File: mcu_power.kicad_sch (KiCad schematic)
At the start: 36 parts, among them U1 MIMXRT1052CVJ5B, Y1 DSC1001BI5-024.0000, Y2 830107834801

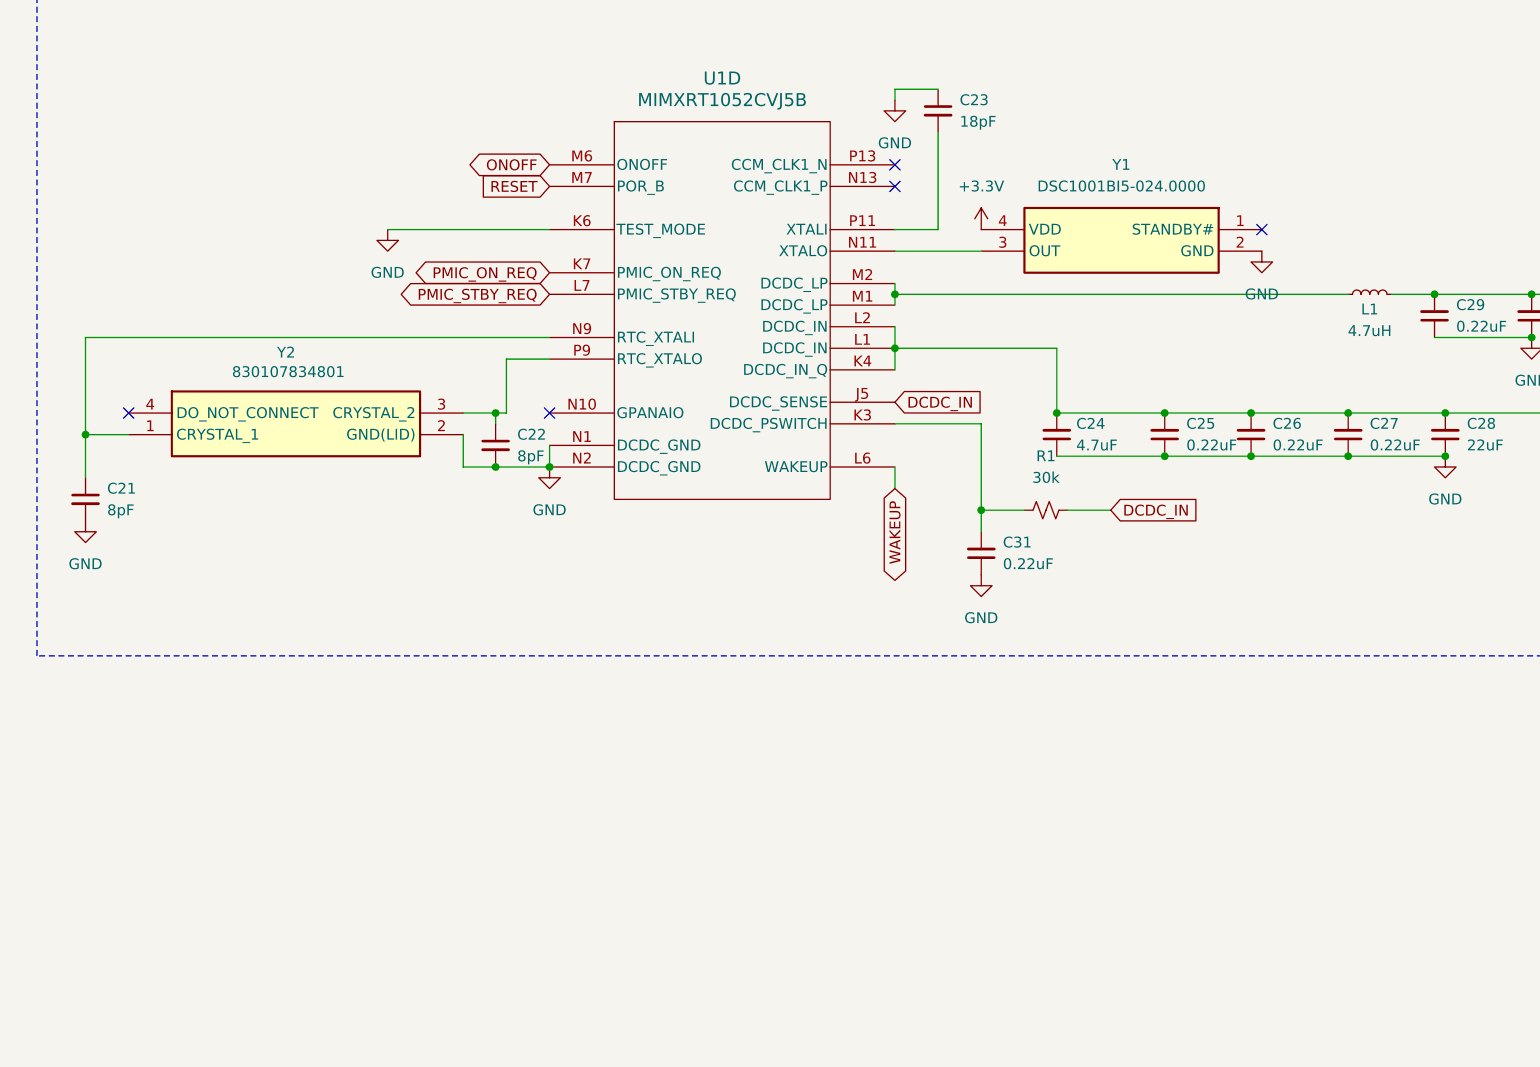
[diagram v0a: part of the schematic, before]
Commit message: v0.2
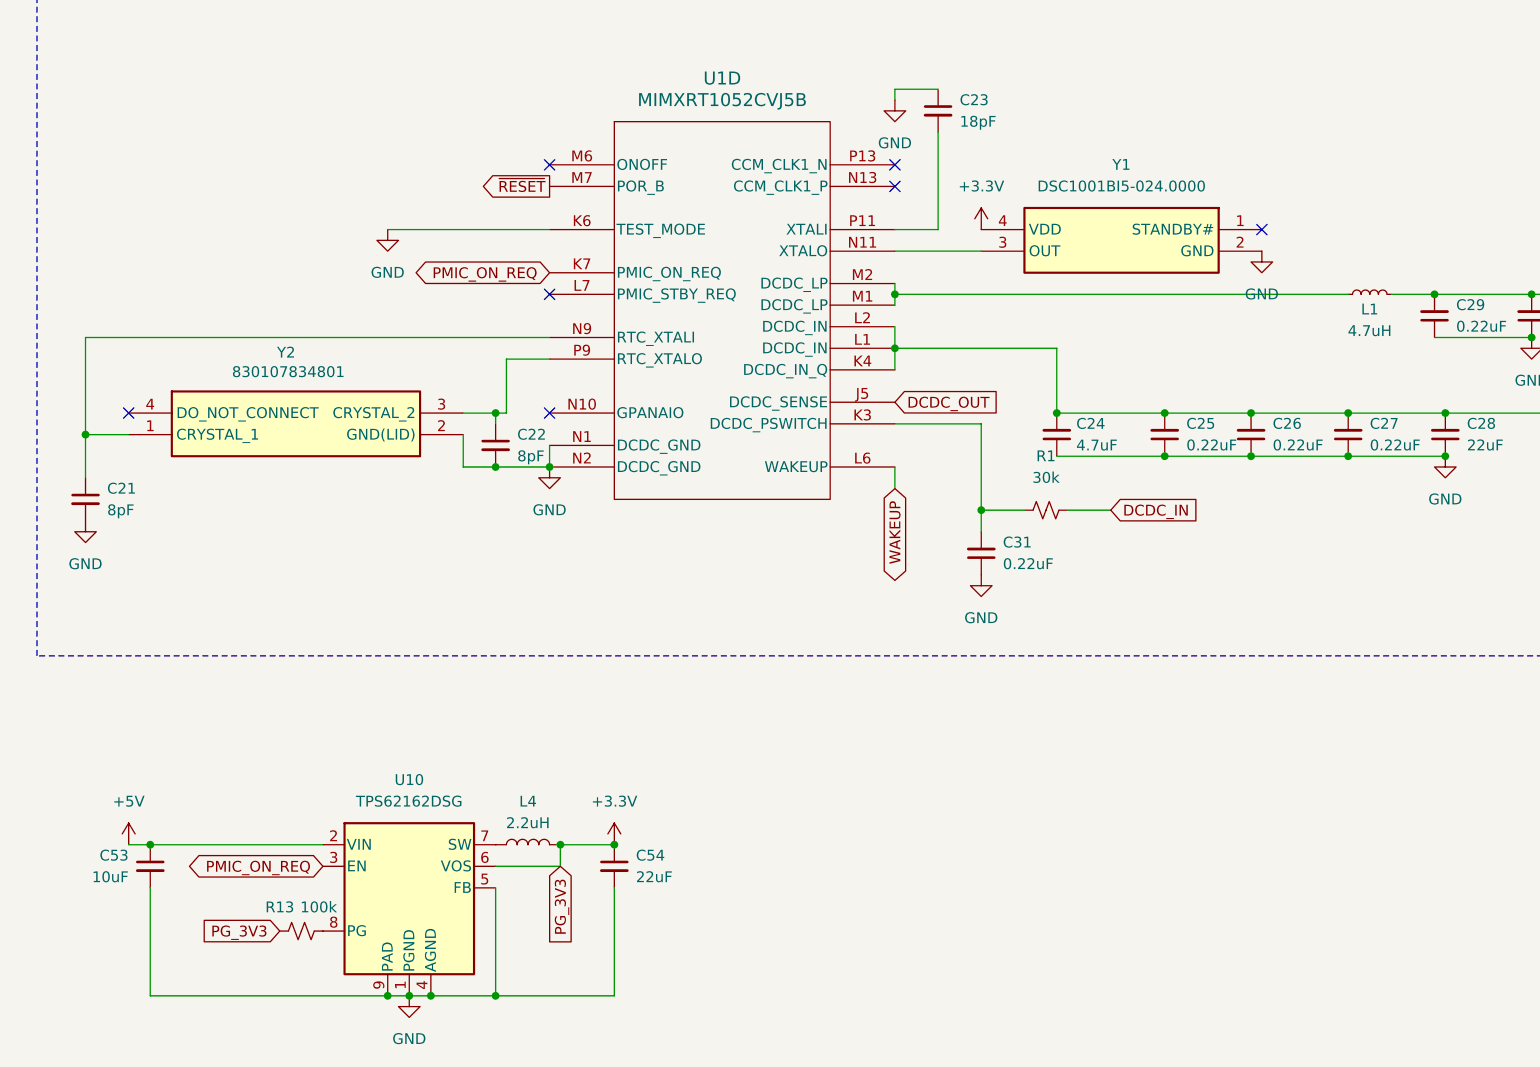
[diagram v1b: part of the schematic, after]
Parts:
- added C53: 10uF, symbol Device:C_Small
- added C54: 22uF, symbol Device:C_Small
- added L4: 2.2uH, symbol Device:L
- added R13: 100k, symbol Device:R_Small_US
- added U10: TPS62162DSG, Package_SON:WSON-8-1EP_2x2mm_P0.5mm_EP0.9x1.6mm_ThermalVias, symbol Regulator_Switching:TPS62162DSG
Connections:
- net +3.3V: now also C54.1, L4.2, R13.1, U10.6 (VOS)
- net DCDC_IN: no longer U1.J5 (DCDC_SENSE)
- net DCDC_OUT: now also U1.J5 (DCDC_SENSE)
- net GND: now also C53.2, C54.2, U10.1 (PGND), U10.4 (AGND), U10.5 (FB), U10.9 (PAD)
- net PMIC_ON_REQ: now also U10.3 (EN)
- net ONOFF: no longer names the net of U1.M6 (ONOFF)
- net PMIC_STBY_REQ: no longer names the net of U1.L7 (PMIC_STBY_REQ)
- net RESET renamed ~{RESET}
- new net: R13.2, U10.8 (PG)
- new net: L4.1, U10.7 (SW)
- new net +5V: C53.1, U10.2 (VIN)
- no-connect marks 5 -> 7
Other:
- title: RT1050 DevBoard for Project Horizon -> Payload Board for Pleiades Atlas
